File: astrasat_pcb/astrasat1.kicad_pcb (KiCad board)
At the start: 2 copper layers, 120 x 120 mm, 28 parts, among them SW1 SW_SPDT, U3 DS1302+, U5 Pico, Y1 Crystal

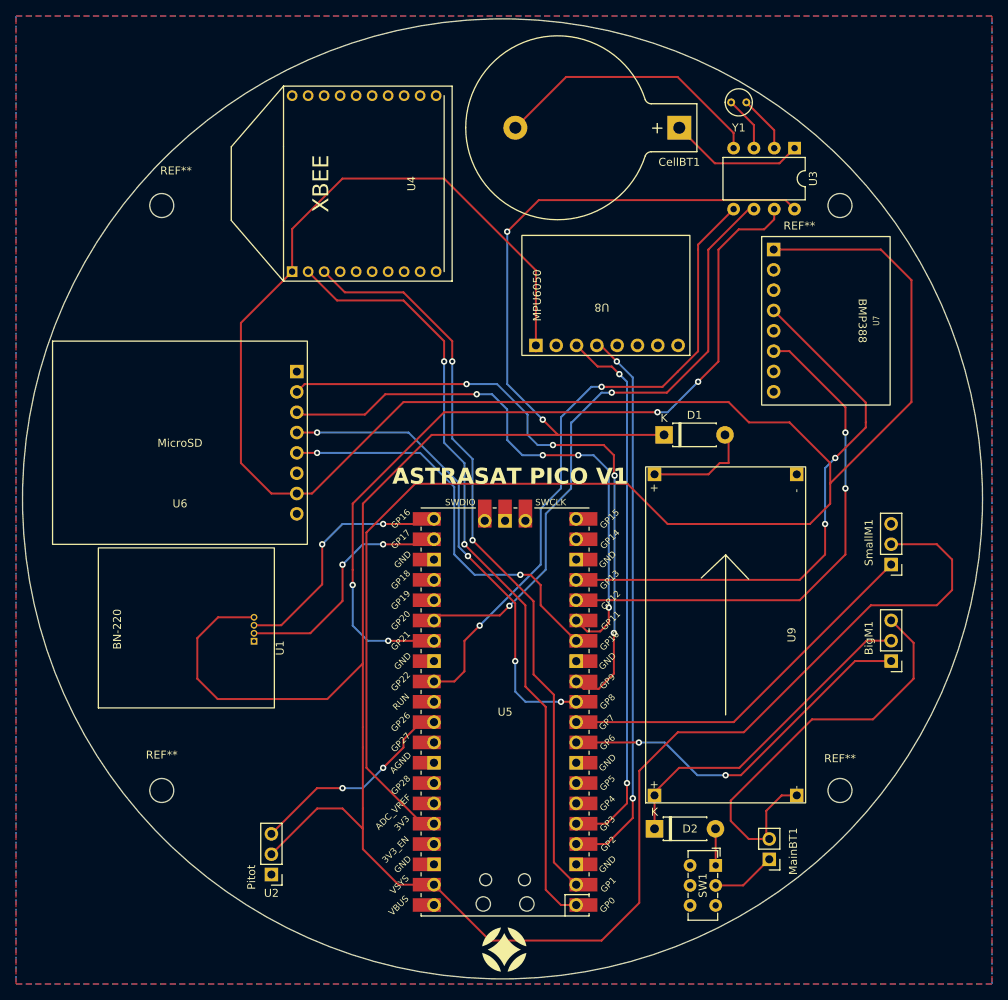
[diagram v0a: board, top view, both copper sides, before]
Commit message: reduce pcb size
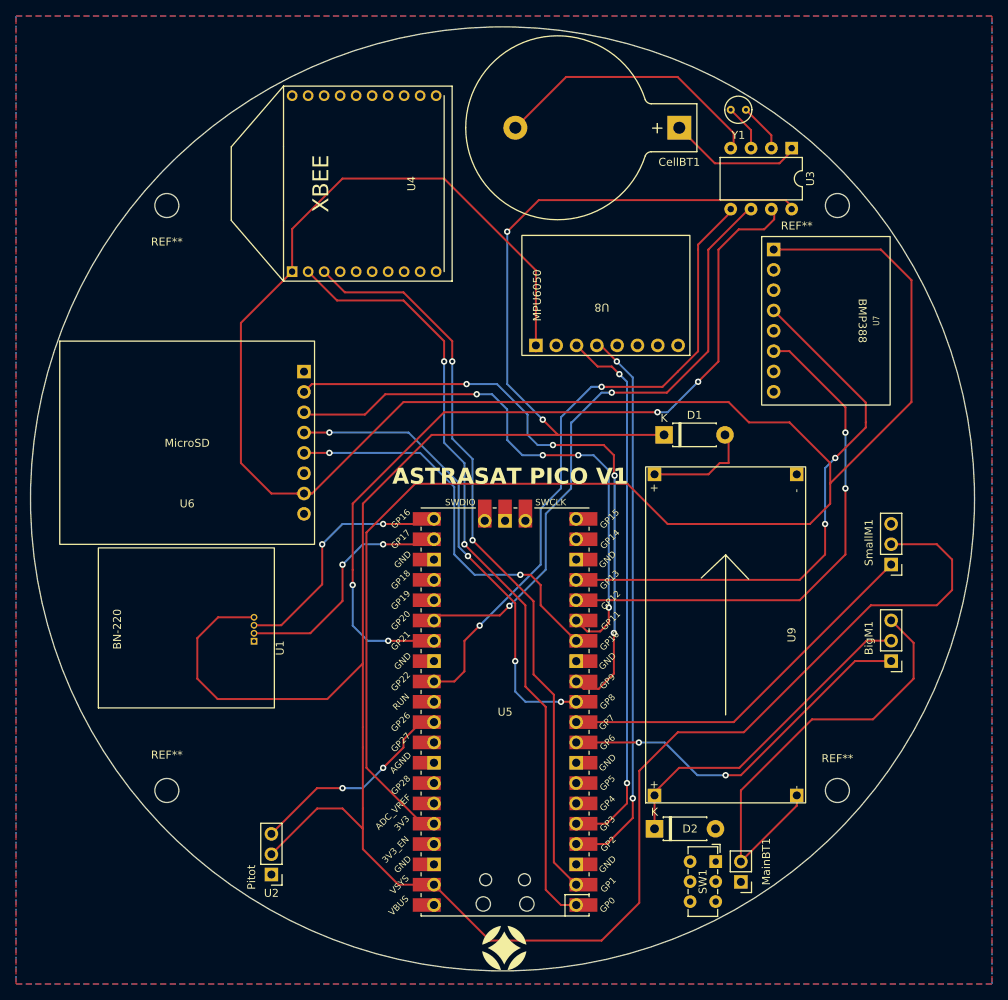
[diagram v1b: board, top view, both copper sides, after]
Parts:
- moved MainBT1 4.53 mm to (181.6, 142.2)
- moved Y1 0.93 mm to (180.3, 45.7)
- moved U6 0.90 mm to (112.4, 87.3)
- moved REF** 0.64 mm to (109.9, 57.7)
- moved REF** 0.64 mm to (109.9, 130.8)
- moved SW1 0.48 mm to (178.5, 139.7)
- moved U3 0.36 mm to (188.0, 50.5)
- moved REF** 0.32 mm to (193.7, 130.8)
- moved REF** 0.32 mm to (193.7, 57.7)
- moved G*** 0.20 mm to (152.0, 150.5)
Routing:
- net Net-(MainBT1-+): track 8.05 -> 0.00 mm
- net Net-(D2-A): track 4.59 -> 0.04 mm
- net GND2: track 54.6 -> 55.9 mm
- net Net-(U3-X1): track 7.17 -> 6.12 mm
- net Net-(U3-X2): track 6.90 -> 5.85 mm
- net /GPIO9: track 78.5 -> 77.6 mm
- net /GPIO11: track 70.5 -> 69.6 mm
- net /GPIO10: track 51.1 -> 50.2 mm
- net /GPIO8: track 60.0 -> 59.1 mm
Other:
- board size 120 x 120 mm -> 118 x 118 mm
